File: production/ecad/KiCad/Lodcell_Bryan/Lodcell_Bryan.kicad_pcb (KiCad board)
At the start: 2 copper layers, 70.6 x 37.9 mm, 26 parts, among them J1 LoadCellConnector, J2 power_for_Loadcell, J3 ConnToESP32, U1 MIC920YC5-TR, U2 MIC920YC5-TR, U3 ADS1231IDR, U4 TXB0104DR

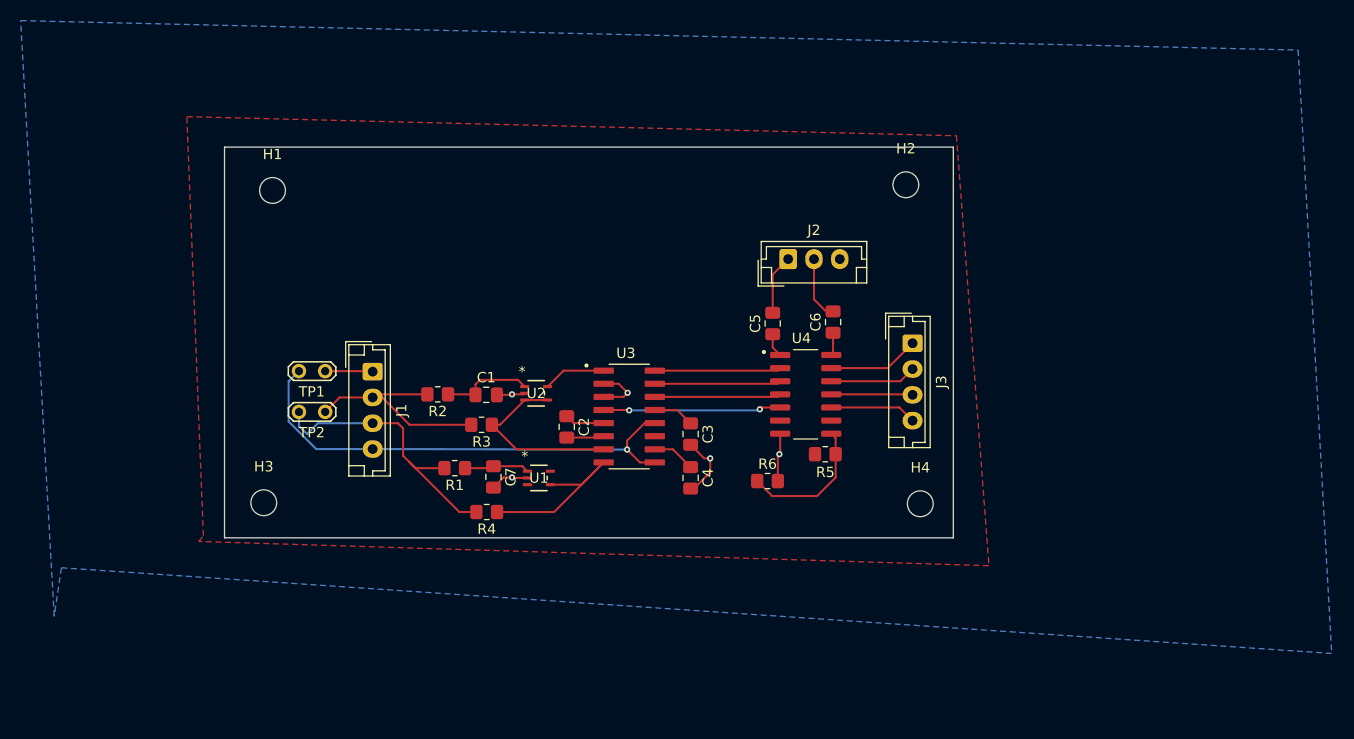
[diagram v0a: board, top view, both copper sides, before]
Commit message: Changes
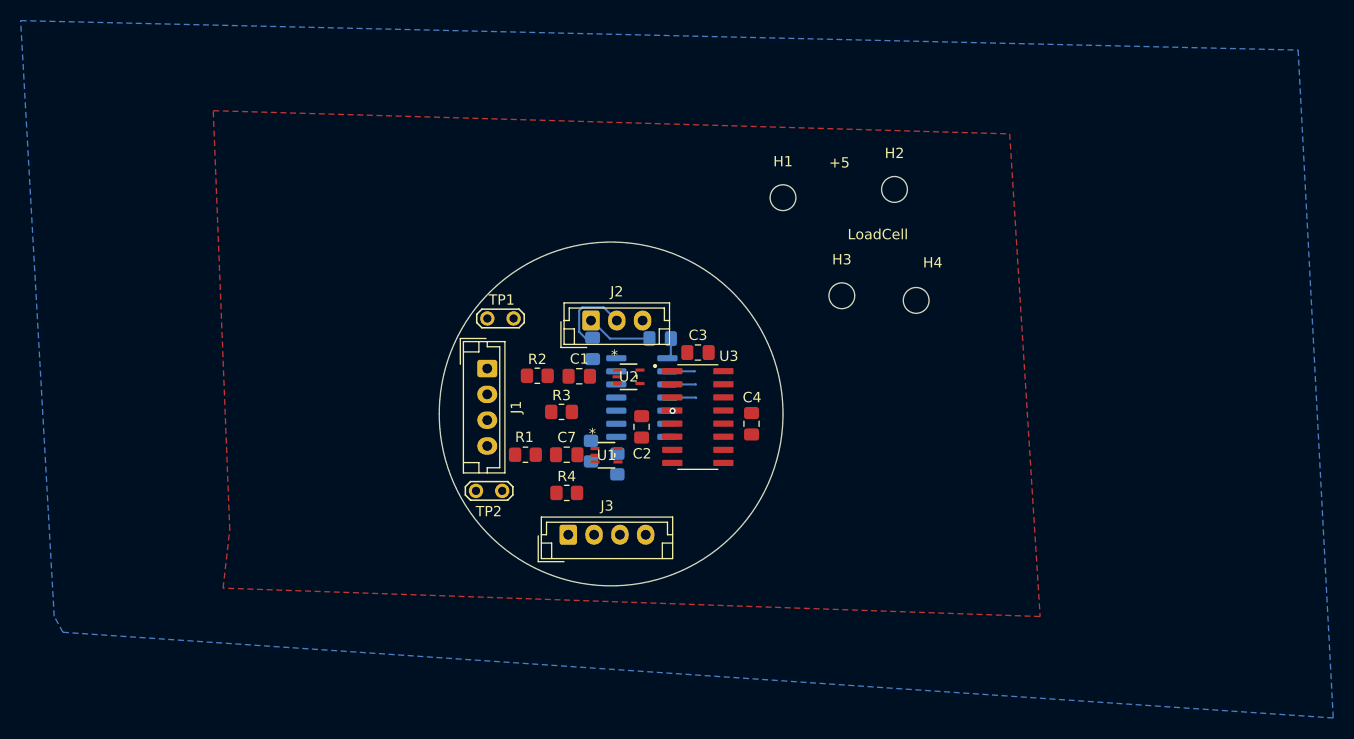
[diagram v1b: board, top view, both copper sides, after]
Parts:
- C5, C6, R5, R6, U4: moved to B.Cu
- moved H3 59.5 mm to (185.0, 55.2)
- moved H1 49.5 mm to (179.3, 45.7)
- moved J3 38.2 mm to (158.5, 78.3), turned to 0 degrees
- moved C6 23.4 mm to (160.8, 60.3)
- moved R5 22.7 mm to (160.7, 70.2), turned to 90 degrees
- moved J2 20.0 mm to (160.7, 57.6)
- moved H4 19.7 mm to (192.2, 55.6)
- moved TP1 18.9 mm to (153.2, 57.4)
- moved TP2 18.8 mm to (152.1, 74.1)
- moved U4 15.9 mm to (165.6, 65.1), turned to 180 degrees
- moved R6 14.6 mm to (163.2, 71.5), turned to -90 degrees
- moved J1 11.1 mm to (150.7, 62.2)
- moved C5 11.0 mm to (167.4, 59.4), turned to 180 degrees
- moved R2 9.82 mm to (155.5, 63.0)
- moved C1 9.19 mm to (159.6, 63.0)
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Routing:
- net Net-(J1-Pin_4): track 46.7 -> 0.00 mm, vias 1 -> 0
- net /RawLoadCell_-: track 28.1 -> 0.00 mm
- net GND: track 22.7 -> 0.00 mm, vias 5 -> 0
- net /RawLoadCell_+: track 21.3 -> 0.00 mm
- net /LP_-: track 18.4 -> 0.00 mm
- net /LP_+: track 18.2 -> 0.00 mm
- net Net-(U3-SPEED): track 17.4 -> 0.00 mm, vias 2 -> 1
- net +5V: track 25.1 -> 7.89 mm
- net Net-(U4-OE): track 13.4 -> 0.00 mm
- net Net-(U3-~{DRDY}/DOUT): track 12.2 -> 2.66 mm
- net Net-(U3-SCLK): track 12.2 -> 2.75 mm
- net Net-(U3-~{PDWN}): track 12.2 -> 2.82 mm
- net Net-(U2-IN+): track 8.91 -> 0.00 mm
- net MISO: track 8.87 -> 0.00 mm
- net Net-(J3-Pin_4): track 8.41 -> 0.00 mm
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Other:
- board size 70.6 x 37.9 mm -> 33.3 x 33.3 mm
- board text added: "+3.3"
- board text added: "+5"
- board text added: "-"
- board text added: "LoadCell"
